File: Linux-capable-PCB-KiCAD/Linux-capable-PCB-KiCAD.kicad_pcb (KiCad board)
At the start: 4 copper layers, 168 parts, among them J1 UART_CONN, J2 GPIO_CONN, J3 USB_A, J4 USB_A, J5 Micro_SD_Card_Det, J6 MIC_DIFF_IN, J7 Barrel_Jack, U1 A33, U10 TPS62130, U11 AP131-25, U12 TPS62130, U13 TPS62130, U2 MMA8425Q_Gsensor, U3 SRV05-4, U4 MIPI_DSI_Raspberry, U5 SRV05-4, U6 SRV05-4, U7 ESP8089, U8 HTQ4G63AFR-PCB, U9 TPS62130, Y1 24MHz, Y2 32.768kHz, Y3 26 MHz

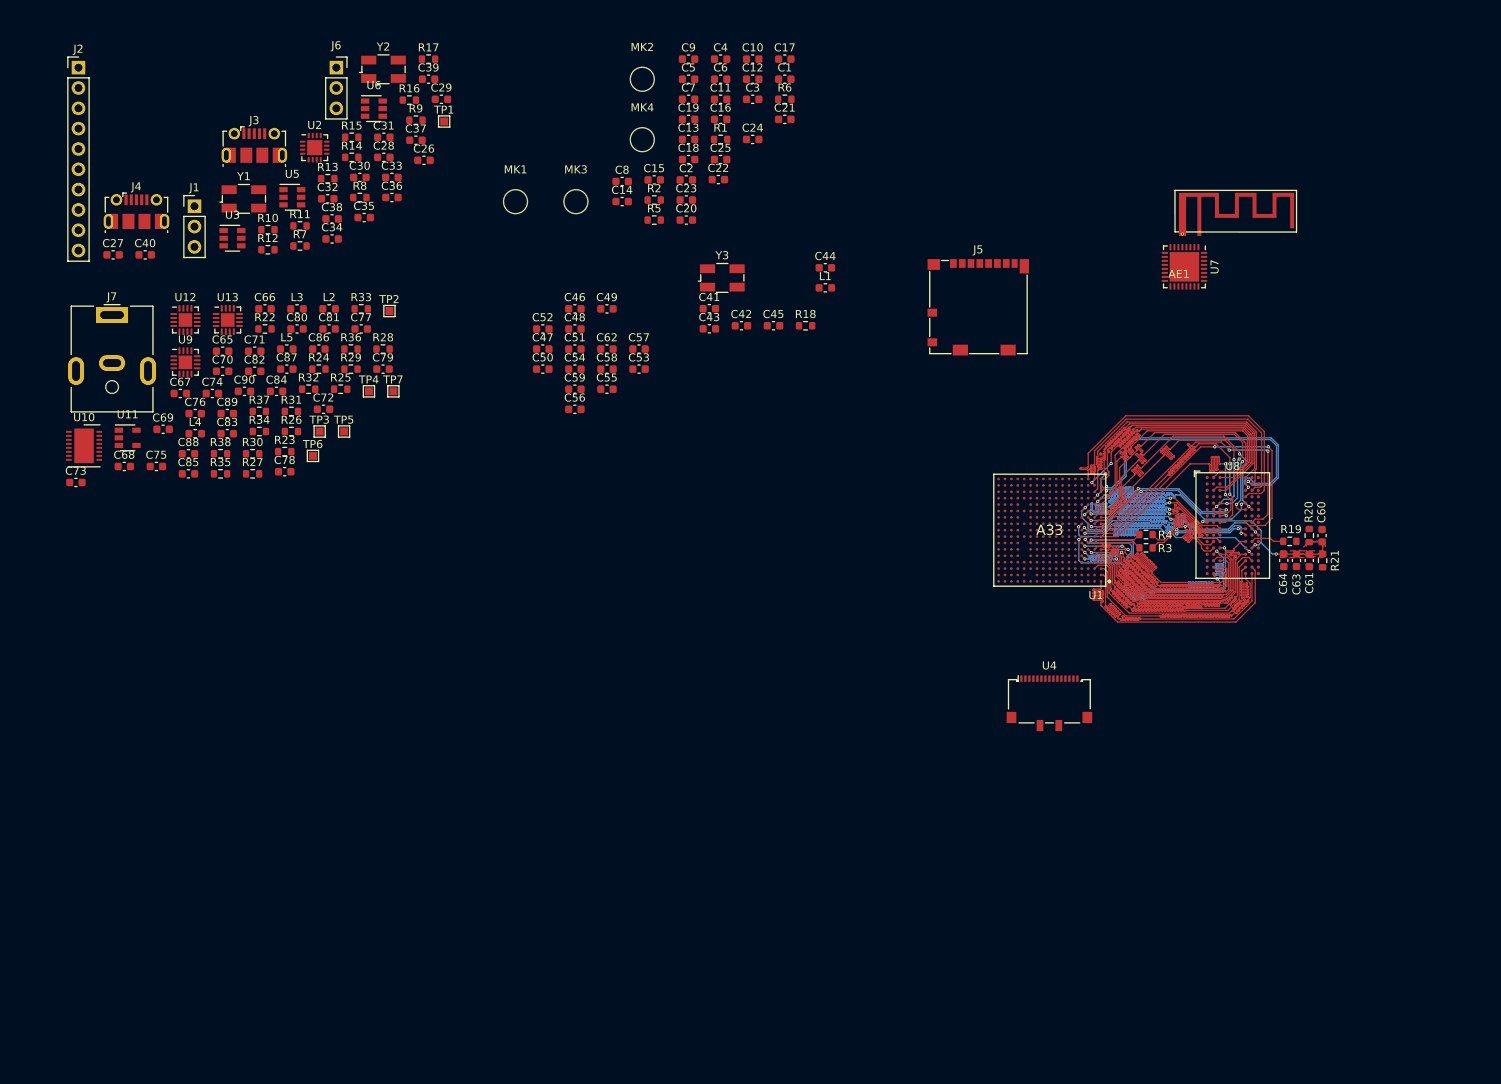
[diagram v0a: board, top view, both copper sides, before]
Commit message: Od kuce
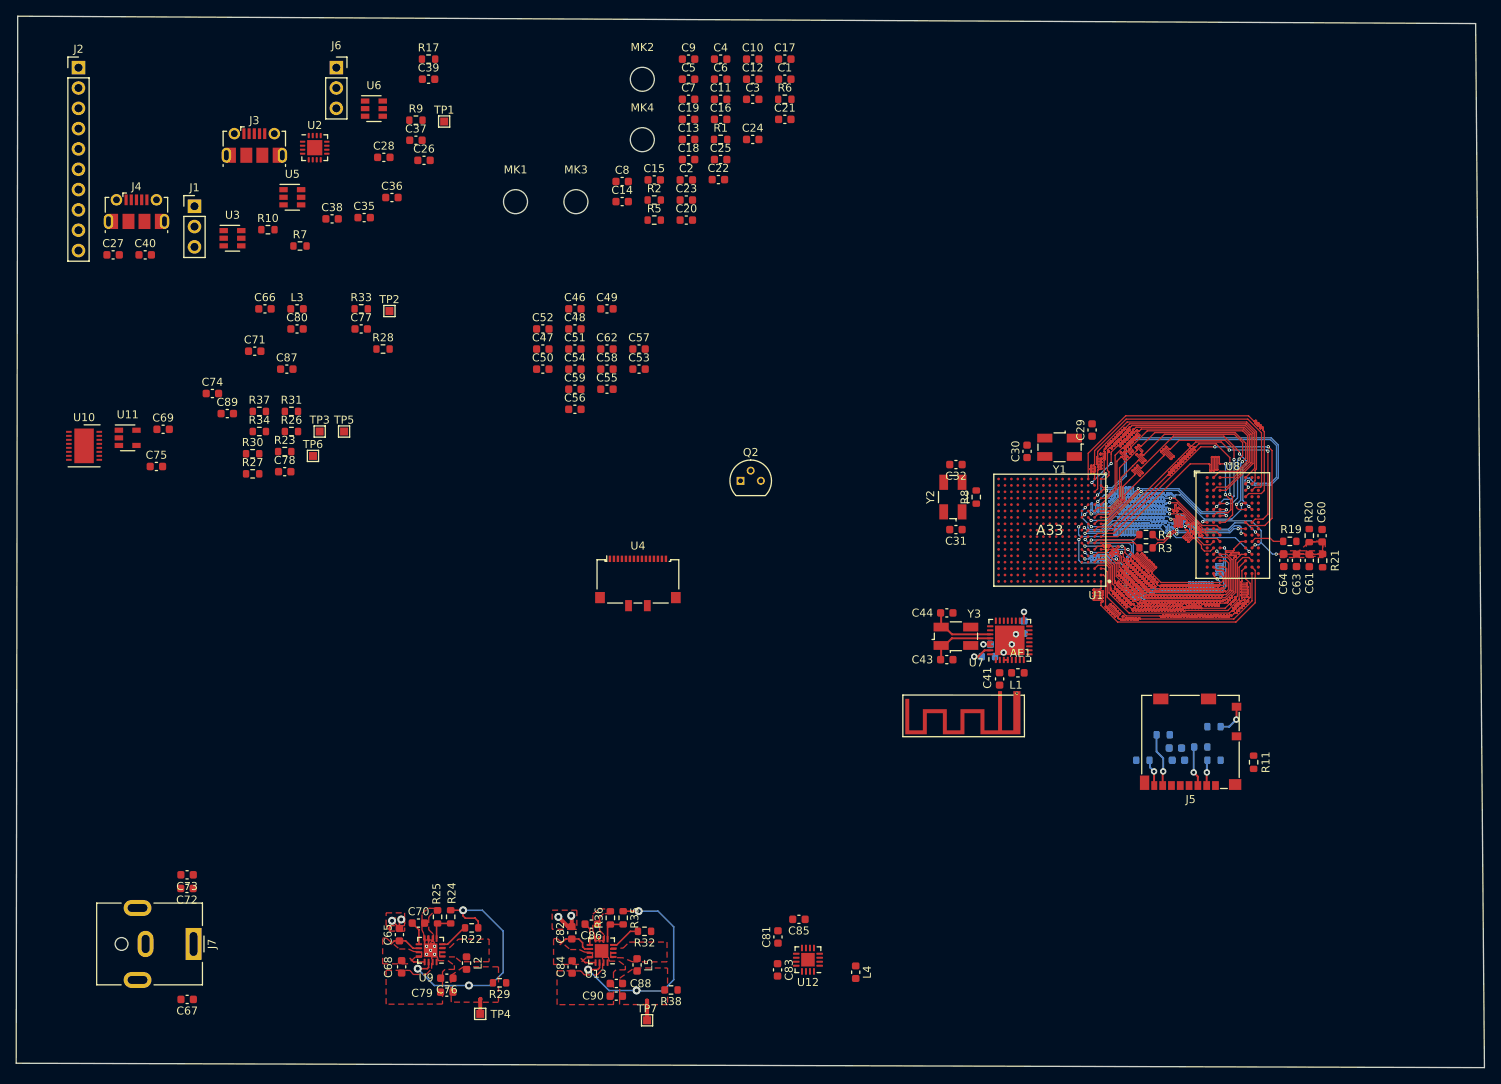
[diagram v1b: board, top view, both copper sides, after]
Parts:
- added Q2: BC547, TO_SOT_Packages_THT:TO-92_Molded_Narrow, F.Cu at (113.8, 72.5)
- C33, C34, C42, C45, R12, R13, R14, R15, R16, R18: moved to B.Cu
- moved R11 136.8 mm to (177.9, 107.7), turned to 90 degrees
- moved R12 134.4 mm to (173.0, 107.4)
- moved R13 130.2 mm to (171.3, 105.8)
- moved R16 127.5 mm to (173.0, 103.3), turned to 180 degrees
- moved R15 125.9 mm to (164.1, 107.4), turned to 180 degrees
- moved R14 124.5 mm to (166.6, 104.3)
- moved C34 124.2 mm to (168.5, 107.4)
- moved C33 121.2 mm to (168.1, 105.9)
- moved U12 111.6 mm to (122.2, 132.4), turned to 180 degrees
- moved Y1 106.6 mm to (153.7, 68.3), turned to 180 degrees
- moved L4 106.5 mm to (128.2, 133.9), turned to -90 degrees
- moved C83 96.0 mm to (118.4, 133.7), turned to -90 degrees
- moved C81 94.5 mm to (118.5, 129.5), turned to 90 degrees
- moved C85 94.5 mm to (121.1, 127.3), turned to 180 degrees
- moved U13 91.7 mm to (96.4, 131.3), turned to 180 degrees
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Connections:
- net /RAM/~CAS renamed /RAM/~{CAS}
- net /RAM/~CKE renamed /RAM/~{CKE}
- net /RAM/~CS renamed /RAM/~{CS}
- net /RAM/~RAS renamed /RAM/~{RAS}
- net /RAM/~RST renamed /RAM/~{RST}
- net /RAM/~WE renamed /RAM/~{WE}
- C29 pad 1: Net-(C29-Pad1) -> unconnected-(C29-Pad1)
- C33 pad 1: Net-(C33-Pad1) -> +3V3
- C34 pad 1: Net-(C33-Pad1) -> +3V3
- J5 pad 4: Net-(C33-Pad1) -> +3V3
- R11 pad 2: Net-(C33-Pad1) -> +3V3
- R12 pad 2: Net-(C33-Pad1) -> +3V3
- R13 pad 2: Net-(C33-Pad1) -> +3V3
- R14 pad 2: Net-(C33-Pad1) -> +3V3
- R15 pad 2: Net-(C33-Pad1) -> +3V3
- R16 pad 2: Net-(C33-Pad1) -> +3V3
- U1 pad A10: Net-(U1-PadA10) -> unconnected-(U1-PadA10)
- U1 pad A11: Net-(U1-PadA11) -> unconnected-(U1-PadA11)
- U1 pad A12: Net-(U1-PadA12) -> unconnected-(U1-PadA12)
- U1 pad A16: Net-(U1-PadA16) -> unconnected-(U1-PadA16)
- U1 pad A2: Net-(U1-PadA2) -> unconnected-(U1-PadA2)
- U1 pad A7: Net-(U1-PadA7) -> unconnected-(U1-PadA7)
- U1 pad A8: Net-(U1-PadA8) -> unconnected-(U1-PadA8)
- U1 pad A9: Net-(U1-PadA9) -> unconnected-(U1-PadA9)
- U1 pad B10: Net-(U1-PadB10) -> unconnected-(U1-PadB10)
- U1 pad B11: Net-(U1-PadB11) -> unconnected-(U1-PadB11)
- U1 pad B16: Net-(U1-PadB16) -> unconnected-(U1-PadB16)
- U1 pad B17: Net-(U1-PadB17) -> unconnected-(U1-PadB17)
- U1 pad B2: Net-(U1-PadB2) -> unconnected-(U1-PadB2)
- U1 pad B7: Net-(U1-PadB7) -> unconnected-(U1-PadB7)
- U1 pad B8: Net-(U1-PadB8) -> unconnected-(U1-PadB8)
- U1 pad B9: Net-(U1-PadB9) -> unconnected-(U1-PadB9)
- U1 pad C10: Net-(U1-PadC10) -> unconnected-(U1-PadC10)
- U1 pad C11: Net-(U1-PadC11) -> unconnected-(U1-PadC11)
- U1 pad C12: Net-(U1-PadC12) -> unconnected-(U1-PadC12)
- U1 pad C13: Net-(U1-PadC13) -> unconnected-(U1-PadC13)
- U1 pad C14: Net-(U1-PadC14) -> unconnected-(U1-PadC14)
- U1 pad C15: Net-(U1-PadC15) -> unconnected-(U1-PadC15)
- U1 pad C16: Net-(U1-PadC16) -> unconnected-(U1-PadC16)
- U1 pad C17: Net-(U1-PadC17) -> unconnected-(U1-PadC17)
- U1 pad C3: Net-(U1-PadC3) -> unconnected-(U1-PadC3)
- U1 pad C4: Net-(U1-PadC4) -> unconnected-(U1-PadC4)
- U1 pad D10: Net-(U1-PadD10) -> unconnected-(U1-PadD10)
- U1 pad D11: Net-(U1-PadD11) -> unconnected-(U1-PadD11)
- U1 pad D12: Net-(U1-PadD12) -> unconnected-(U1-PadD12)
- U1 pad D13: Net-(U1-PadD13) -> unconnected-(U1-PadD13)
- U1 pad D3: Net-(U1-PadD3) -> unconnected-(U1-PadD3)
- U1 pad D4: Net-(U1-PadD4) -> unconnected-(U1-PadD4)
- U1 pad E14: Net-(U1-PadE14) -> unconnected-(U1-PadE14)
- U1 pad E15: Net-(U1-PadE15) -> unconnected-(U1-PadE15)
- U1 pad E16: Net-(U1-PadE16) -> unconnected-(U1-PadE16)
- U1 pad E17: Net-(U1-PadE17) -> unconnected-(U1-PadE17)
- U1 pad F14: Net-(U1-PadF14) -> unconnected-(U1-PadF14)
- U1 pad F15: Net-(U1-PadF15) -> unconnected-(U1-PadF15)
- U1 pad F16: Net-(U1-PadF16) -> unconnected-(U1-PadF16)
- U1 pad F17: Net-(U1-PadF17) -> unconnected-(U1-PadF17)
- U1 pad G15: Net-(U1-PadG15) -> unconnected-(U1-PadG15)
- U1 pad H14: Net-(U1-PadH14) -> unconnected-(U1-PadH14)
- U1 pad H15: Net-(U1-PadH15) -> unconnected-(U1-PadH15)
- U1 pad H16: Net-(U1-PadH16) -> unconnected-(U1-PadH16)
- U1 pad J14: Net-(U1-PadJ14) -> unconnected-(U1-PadJ14)
- U1 pad J15: Net-(U1-PadJ15) -> unconnected-(U1-PadJ15)
- U1 pad J16: Net-(U1-PadJ16) -> unconnected-(U1-PadJ16)
- U1 pad J17: Net-(U1-PadJ17) -> unconnected-(U1-PadJ17)
- U1 pad K14: Net-(U1-PadK14) -> unconnected-(U1-PadK14)
- U1 pad K15: Net-(U1-PadK15) -> unconnected-(U1-PadK15)
- U1 pad L14: Net-(U1-PadL14) -> unconnected-(U1-PadL14)
- U1 pad L15: Net-(U1-PadL15) -> unconnected-(U1-PadL15)
- U1 pad L7: Net-(U1-PadL7) -> unconnected-(U1-PadL7)
- U1 pad M1: d0 -> d[0..15]
- U1 pad M15: Net-(U1-PadM15) -> unconnected-(U1-PadM15)
- U1 pad N15: Net-(U1-PadN15) -> unconnected-(U1-PadN15)
- U1 pad N16: Net-(U1-PadN16) -> unconnected-(U1-PadN16)
- U1 pad N17: Net-(U1-PadN17) -> unconnected-(U1-PadN17)
- U1 pad N5: Net-(U1-PadN5) -> unconnected-(U1-PadN5)
- U1 pad N7: Net-(U1-PadN7) -> unconnected-(U1-PadN7)
- U1 pad P10: Net-(U1-PadP10) -> unconnected-(U1-PadP10)
- U1 pad P11: Net-(U1-PadP11) -> unconnected-(U1-PadP11)
- U1 pad P12: Net-(U1-PadP12) -> unconnected-(U1-PadP12)
- U1 pad P13: Net-(U1-PadP13) -> unconnected-(U1-PadP13)
- U1 pad P14: Net-(U1-PadP14) -> unconnected-(U1-PadP14)
- U1 pad P15: Net-(U1-PadP15) -> unconnected-(U1-PadP15)
- U1 pad P16: Net-(U1-PadP16) -> unconnected-(U1-PadP16)
- U1 pad P6: Net-(U1-PadP6) -> unconnected-(U1-PadP6)
- U1 pad P7: Net-(U1-PadP7) -> unconnected-(U1-PadP7)
- U1 pad P8: Net-(U1-PadP8) -> unconnected-(U1-PadP8)
- U1 pad P9: Net-(U1-PadP9) -> unconnected-(U1-PadP9)
- U1 pad R10: Net-(U1-PadR10) -> unconnected-(U1-PadR10)
- U1 pad R11: Net-(U1-PadR11) -> unconnected-(U1-PadR11)
- U1 pad R12: Net-(U1-PadR12) -> unconnected-(U1-PadR12)
- U1 pad R13: Net-(U1-PadR13) -> unconnected-(U1-PadR13)
- U1 pad R14: Net-(U1-PadR14) -> unconnected-(U1-PadR14)
- U1 pad R15: Net-(U1-PadR15) -> unconnected-(U1-PadR15)
- U1 pad R6: Net-(U1-PadR6) -> unconnected-(U1-PadR6)
- U1 pad R7: Net-(U1-PadR7) -> unconnected-(U1-PadR7)
- U1 pad R8: Net-(U1-PadR8) -> unconnected-(U1-PadR8)
- U1 pad R9: Net-(U1-PadR9) -> unconnected-(U1-PadR9)
- U1 pad T10: Net-(U1-PadT10) -> unconnected-(U1-PadT10)
- U1 pad T11: Net-(U1-PadT11) -> unconnected-(U1-PadT11)
- U1 pad T12: Net-(U1-PadT12) -> unconnected-(U1-PadT12)
- U1 pad T13: Net-(U1-PadT13) -> unconnected-(U1-PadT13)
- U1 pad T14: Net-(U1-PadT14) -> unconnected-(U1-PadT14)
- U1 pad T15: Net-(U1-PadT15) -> unconnected-(U1-PadT15)
- U1 pad T6: Net-(U1-PadT6) -> unconnected-(U1-PadT6)
- U1 pad T7: Net-(U1-PadT7) -> unconnected-(U1-PadT7)
- U1 pad T8: Net-(U1-PadT8) -> unconnected-(U1-PadT8)
- U1 pad T9: Net-(U1-PadT9) -> unconnected-(U1-PadT9)
- U1 pad U10: Net-(U1-PadU10) -> unconnected-(U1-PadU10)
- U1 pad U11: Net-(U1-PadU11) -> unconnected-(U1-PadU11)
- U1 pad U12: Net-(U1-PadU12) -> unconnected-(U1-PadU12)
- U1 pad U13: /A33_GPIO/VBUS_~EN -> /A33_GPIO/VBUS_~{EN}
- U1 pad U14: Net-(U1-PadU14) -> unconnected-(U1-PadU14)
- U1 pad U15: Net-(U1-PadU15) -> unconnected-(U1-PadU15)
- U1 pad U6: Net-(U1-PadU6) -> unconnected-(U1-PadU6)
- U1 pad U7: Net-(U1-PadU7) -> unconnected-(U1-PadU7)
- U1 pad U8: Net-(U1-PadU8) -> unconnected-(U1-PadU8)
- U1 pad U9: Net-(U1-PadU9) -> unconnected-(U1-PadU9)
- U2 pad 13: Net-(U2-Pad13) -> unconnected-(U2-Pad13)
- U2 pad 15: Net-(U2-Pad15) -> unconnected-(U2-Pad15)
- U2 pad 16: Net-(U2-Pad16) -> unconnected-(U2-Pad16)
- U2 pad 3: Net-(U2-Pad3) -> unconnected-(U2-Pad3)
- U2 pad 8: Net-(U2-Pad8) -> unconnected-(U2-Pad8)
- U7 pad 10: Net-(U7-Pad10) -> unconnected-(U7-Pad10)
- U7 pad 12: Net-(U7-Pad12) -> unconnected-(U7-Pad12)
- U7 pad 13: Net-(U7-Pad13) -> unconnected-(U7-Pad13)
- U7 pad 14: Net-(U7-Pad14) -> unconnected-(U7-Pad14)
- U7 pad 15: Net-(U7-Pad15) -> unconnected-(U7-Pad15)
- U7 pad 16: Net-(U7-Pad16) -> unconnected-(U7-Pad16)
- U7 pad 24: Net-(U7-Pad24) -> unconnected-(U7-Pad24)
- U7 pad 25: Net-(U7-Pad25) -> unconnected-(U7-Pad25)
- U7 pad 26: Net-(U7-Pad26) -> unconnected-(U7-Pad26)
- U7 pad 32: Net-(U7-Pad32) -> unconnected-(U7-Pad32)
- U7 pad 5: Net-(U7-Pad5) -> unconnected-(U7-Pad5)
- U7 pad 6: Net-(U7-Pad6) -> unconnected-(U7-Pad6)
- U7 pad 8: Net-(U7-Pad8) -> unconnected-(U7-Pad8)
- U7 pad 9: Net-(U7-Pad9) -> unconnected-(U7-Pad9)
- U8 pad J1: Net-(U8-PadJ1) -> unconnected-(U8-PadJ1)
- U8 pad J9: Net-(U8-PadJ9) -> unconnected-(U8-PadJ9)
- U8 pad L1: Net-(U8-PadL1) -> unconnected-(U8-PadL1)
- U8 pad L9: Net-(U8-PadL9) -> unconnected-(U8-PadL9)
- U8 pad M7: Net-(U8-PadM7) -> unconnected-(U8-PadM7)
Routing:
- net d[0..15]: track 0.00 -> 38.0 mm, vias 0 -> 2
- net d0: track 38.0 -> 0.00 mm, vias 2 -> 0
- net Net-(C76-Pad1): track 0.00 -> 32.8 mm, vias 0 -> 3
- net Net-(C88-Pad1): track 0.00 -> 30.8 mm, vias 0 -> 3
- net GND: track 0.00 -> 19.0 mm, vias 0 -> 12
- net +5V: track 0.00 -> 12.9 mm
- net Net-(C44-Pad2): track 0.00 -> 8.31 mm
- net Net-(C43-Pad2): track 0.00 -> 8.30 mm
- net /A33_GPIO/SD_DAT0: track 0.00 -> 6.71 mm, vias 0 -> 1
- net /A33_GPIO/SD_CMD: track 0.00 -> 5.06 mm, vias 0 -> 1
- net +3V3: track 0.00 -> 4.99 mm, vias 0 -> 2
- net /A33_GPIO/SD_DET: track 0.00 -> 3.95 mm, vias 0 -> 1
- net Net-(R32-Pad2): track 0.00 -> 3.79 mm
- net Net-(R22-Pad2): track 0.00 -> 3.69 mm
- net Net-(R35-Pad2): track 0.00 -> 3.62 mm
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- added copper zone on F.Cu, net +5V
- added copper zone on F.Cu, net GND
- added copper zone on F.Cu, net Net-(C76-Pad1)
- added copper zone on F.Cu, net Net-(C88-Pad1)
- added copper zone on F.Cu, net Net-(L2-Pad1)
- added copper zone on F.Cu, net Net-(L5-Pad1)
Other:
- board outline added: 183.5 x 131.4 mm
- net class Default removed
- net class Outer_small removed
- net class Power removed

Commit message: Revert "Od kuce"
This reverts commit 2bece482254f98a379437a0618b8cb6327aa6629.
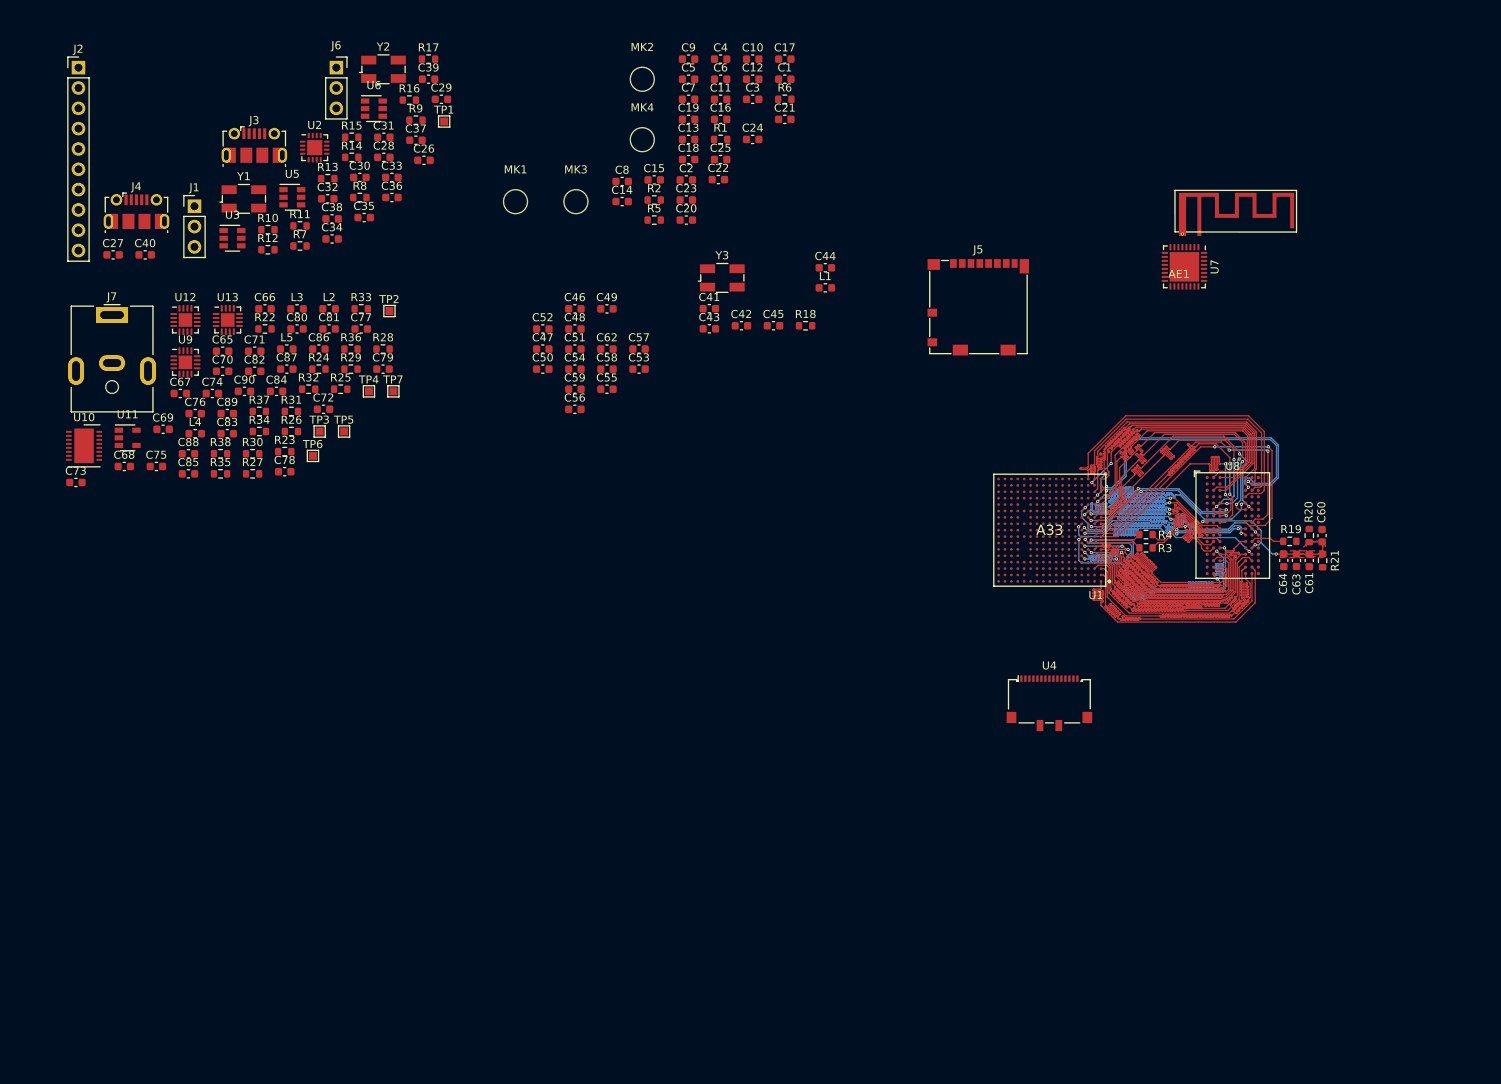
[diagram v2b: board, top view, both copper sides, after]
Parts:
- removed Q2: BC547, TO_SOT_Packages_THT:TO-92_Molded_Narrow
- C33, C34, C42, C45, R12, R13, R14, R15, R16, R18: moved to F.Cu
- moved R11 136.8 mm to (58.7, 40.7), turned to 0 degrees
- moved R12 134.4 mm to (54.7, 43.6)
- moved R13 130.2 mm to (62.2, 34.8)
- moved R16 127.5 mm to (72.4, 24.9), turned to 0 degrees
- moved R15 125.9 mm to (65.2, 29.6), turned to 0 degrees
- moved R14 124.5 mm to (65.2, 32.1)
- moved C34 124.2 mm to (62.7, 42.3)
- moved C33 121.2 mm to (70.2, 34.6)
- moved U12 111.6 mm to (44.4, 52.4), turned to 0 degrees
- moved Y1 106.6 mm to (51.7, 37.3), turned to 0 degrees
- moved L4 106.5 mm to (45.6, 66.6), turned to 0 degrees
- moved C83 96.0 mm to (49.6, 66.6), turned to 0 degrees
- moved C81 94.5 mm to (62.4, 53.5), turned to 0 degrees
- moved C85 94.5 mm to (44.8, 71.6), turned to 0 degrees
- moved U13 91.7 mm to (49.7, 52.4), turned to 0 degrees
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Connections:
- net /RAM/~{CAS} renamed /RAM/~CAS
- net /RAM/~{CKE} renamed /RAM/~CKE
- net /RAM/~{CS} renamed /RAM/~CS
- net /RAM/~{RAS} renamed /RAM/~RAS
- net /RAM/~{RST} renamed /RAM/~RST
- net /RAM/~{WE} renamed /RAM/~WE
- C29 pad 1: unconnected-(C29-Pad1) -> Net-(C29-Pad1)
- C33 pad 1: +3V3 -> Net-(C33-Pad1)
- C34 pad 1: +3V3 -> Net-(C33-Pad1)
- J5 pad 4: +3V3 -> Net-(C33-Pad1)
- R11 pad 2: +3V3 -> Net-(C33-Pad1)
- R12 pad 2: +3V3 -> Net-(C33-Pad1)
- R13 pad 2: +3V3 -> Net-(C33-Pad1)
- R14 pad 2: +3V3 -> Net-(C33-Pad1)
- R15 pad 2: +3V3 -> Net-(C33-Pad1)
- R16 pad 2: +3V3 -> Net-(C33-Pad1)
- U1 pad A10: unconnected-(U1-PadA10) -> Net-(U1-PadA10)
- U1 pad A11: unconnected-(U1-PadA11) -> Net-(U1-PadA11)
- U1 pad A12: unconnected-(U1-PadA12) -> Net-(U1-PadA12)
- U1 pad A16: unconnected-(U1-PadA16) -> Net-(U1-PadA16)
- U1 pad A2: unconnected-(U1-PadA2) -> Net-(U1-PadA2)
- U1 pad A7: unconnected-(U1-PadA7) -> Net-(U1-PadA7)
- U1 pad A8: unconnected-(U1-PadA8) -> Net-(U1-PadA8)
- U1 pad A9: unconnected-(U1-PadA9) -> Net-(U1-PadA9)
- U1 pad B10: unconnected-(U1-PadB10) -> Net-(U1-PadB10)
- U1 pad B11: unconnected-(U1-PadB11) -> Net-(U1-PadB11)
- U1 pad B16: unconnected-(U1-PadB16) -> Net-(U1-PadB16)
- U1 pad B17: unconnected-(U1-PadB17) -> Net-(U1-PadB17)
- U1 pad B2: unconnected-(U1-PadB2) -> Net-(U1-PadB2)
- U1 pad B7: unconnected-(U1-PadB7) -> Net-(U1-PadB7)
- U1 pad B8: unconnected-(U1-PadB8) -> Net-(U1-PadB8)
- U1 pad B9: unconnected-(U1-PadB9) -> Net-(U1-PadB9)
- U1 pad C10: unconnected-(U1-PadC10) -> Net-(U1-PadC10)
- U1 pad C11: unconnected-(U1-PadC11) -> Net-(U1-PadC11)
- U1 pad C12: unconnected-(U1-PadC12) -> Net-(U1-PadC12)
- U1 pad C13: unconnected-(U1-PadC13) -> Net-(U1-PadC13)
- U1 pad C14: unconnected-(U1-PadC14) -> Net-(U1-PadC14)
- U1 pad C15: unconnected-(U1-PadC15) -> Net-(U1-PadC15)
- U1 pad C16: unconnected-(U1-PadC16) -> Net-(U1-PadC16)
- U1 pad C17: unconnected-(U1-PadC17) -> Net-(U1-PadC17)
- U1 pad C3: unconnected-(U1-PadC3) -> Net-(U1-PadC3)
- U1 pad C4: unconnected-(U1-PadC4) -> Net-(U1-PadC4)
- U1 pad D10: unconnected-(U1-PadD10) -> Net-(U1-PadD10)
- U1 pad D11: unconnected-(U1-PadD11) -> Net-(U1-PadD11)
- U1 pad D12: unconnected-(U1-PadD12) -> Net-(U1-PadD12)
- U1 pad D13: unconnected-(U1-PadD13) -> Net-(U1-PadD13)
- U1 pad D3: unconnected-(U1-PadD3) -> Net-(U1-PadD3)
- U1 pad D4: unconnected-(U1-PadD4) -> Net-(U1-PadD4)
- U1 pad E14: unconnected-(U1-PadE14) -> Net-(U1-PadE14)
- U1 pad E15: unconnected-(U1-PadE15) -> Net-(U1-PadE15)
- U1 pad E16: unconnected-(U1-PadE16) -> Net-(U1-PadE16)
- U1 pad E17: unconnected-(U1-PadE17) -> Net-(U1-PadE17)
- U1 pad F14: unconnected-(U1-PadF14) -> Net-(U1-PadF14)
- U1 pad F15: unconnected-(U1-PadF15) -> Net-(U1-PadF15)
- U1 pad F16: unconnected-(U1-PadF16) -> Net-(U1-PadF16)
- U1 pad F17: unconnected-(U1-PadF17) -> Net-(U1-PadF17)
- U1 pad G15: unconnected-(U1-PadG15) -> Net-(U1-PadG15)
- U1 pad H14: unconnected-(U1-PadH14) -> Net-(U1-PadH14)
- U1 pad H15: unconnected-(U1-PadH15) -> Net-(U1-PadH15)
- U1 pad H16: unconnected-(U1-PadH16) -> Net-(U1-PadH16)
- U1 pad J14: unconnected-(U1-PadJ14) -> Net-(U1-PadJ14)
- U1 pad J15: unconnected-(U1-PadJ15) -> Net-(U1-PadJ15)
- U1 pad J16: unconnected-(U1-PadJ16) -> Net-(U1-PadJ16)
- U1 pad J17: unconnected-(U1-PadJ17) -> Net-(U1-PadJ17)
- U1 pad K14: unconnected-(U1-PadK14) -> Net-(U1-PadK14)
- U1 pad K15: unconnected-(U1-PadK15) -> Net-(U1-PadK15)
- U1 pad L14: unconnected-(U1-PadL14) -> Net-(U1-PadL14)
- U1 pad L15: unconnected-(U1-PadL15) -> Net-(U1-PadL15)
- U1 pad L7: unconnected-(U1-PadL7) -> Net-(U1-PadL7)
- U1 pad M1: d[0..15] -> d0
- U1 pad M15: unconnected-(U1-PadM15) -> Net-(U1-PadM15)
- U1 pad N15: unconnected-(U1-PadN15) -> Net-(U1-PadN15)
- U1 pad N16: unconnected-(U1-PadN16) -> Net-(U1-PadN16)
- U1 pad N17: unconnected-(U1-PadN17) -> Net-(U1-PadN17)
- U1 pad N5: unconnected-(U1-PadN5) -> Net-(U1-PadN5)
- U1 pad N7: unconnected-(U1-PadN7) -> Net-(U1-PadN7)
- U1 pad P10: unconnected-(U1-PadP10) -> Net-(U1-PadP10)
- U1 pad P11: unconnected-(U1-PadP11) -> Net-(U1-PadP11)
- U1 pad P12: unconnected-(U1-PadP12) -> Net-(U1-PadP12)
- U1 pad P13: unconnected-(U1-PadP13) -> Net-(U1-PadP13)
- U1 pad P14: unconnected-(U1-PadP14) -> Net-(U1-PadP14)
- U1 pad P15: unconnected-(U1-PadP15) -> Net-(U1-PadP15)
- U1 pad P16: unconnected-(U1-PadP16) -> Net-(U1-PadP16)
- U1 pad P6: unconnected-(U1-PadP6) -> Net-(U1-PadP6)
- U1 pad P7: unconnected-(U1-PadP7) -> Net-(U1-PadP7)
- U1 pad P8: unconnected-(U1-PadP8) -> Net-(U1-PadP8)
- U1 pad P9: unconnected-(U1-PadP9) -> Net-(U1-PadP9)
- U1 pad R10: unconnected-(U1-PadR10) -> Net-(U1-PadR10)
- U1 pad R11: unconnected-(U1-PadR11) -> Net-(U1-PadR11)
- U1 pad R12: unconnected-(U1-PadR12) -> Net-(U1-PadR12)
- U1 pad R13: unconnected-(U1-PadR13) -> Net-(U1-PadR13)
- U1 pad R14: unconnected-(U1-PadR14) -> Net-(U1-PadR14)
- U1 pad R15: unconnected-(U1-PadR15) -> Net-(U1-PadR15)
- U1 pad R6: unconnected-(U1-PadR6) -> Net-(U1-PadR6)
- U1 pad R7: unconnected-(U1-PadR7) -> Net-(U1-PadR7)
- U1 pad R8: unconnected-(U1-PadR8) -> Net-(U1-PadR8)
- U1 pad R9: unconnected-(U1-PadR9) -> Net-(U1-PadR9)
- U1 pad T10: unconnected-(U1-PadT10) -> Net-(U1-PadT10)
- U1 pad T11: unconnected-(U1-PadT11) -> Net-(U1-PadT11)
- U1 pad T12: unconnected-(U1-PadT12) -> Net-(U1-PadT12)
- U1 pad T13: unconnected-(U1-PadT13) -> Net-(U1-PadT13)
- U1 pad T14: unconnected-(U1-PadT14) -> Net-(U1-PadT14)
- U1 pad T15: unconnected-(U1-PadT15) -> Net-(U1-PadT15)
- U1 pad T6: unconnected-(U1-PadT6) -> Net-(U1-PadT6)
- U1 pad T7: unconnected-(U1-PadT7) -> Net-(U1-PadT7)
- U1 pad T8: unconnected-(U1-PadT8) -> Net-(U1-PadT8)
- U1 pad T9: unconnected-(U1-PadT9) -> Net-(U1-PadT9)
- U1 pad U10: unconnected-(U1-PadU10) -> Net-(U1-PadU10)
- U1 pad U11: unconnected-(U1-PadU11) -> Net-(U1-PadU11)
- U1 pad U12: unconnected-(U1-PadU12) -> Net-(U1-PadU12)
- U1 pad U13: /A33_GPIO/VBUS_~{EN} -> /A33_GPIO/VBUS_~EN
- U1 pad U14: unconnected-(U1-PadU14) -> Net-(U1-PadU14)
- U1 pad U15: unconnected-(U1-PadU15) -> Net-(U1-PadU15)
- U1 pad U6: unconnected-(U1-PadU6) -> Net-(U1-PadU6)
- U1 pad U7: unconnected-(U1-PadU7) -> Net-(U1-PadU7)
- U1 pad U8: unconnected-(U1-PadU8) -> Net-(U1-PadU8)
- U1 pad U9: unconnected-(U1-PadU9) -> Net-(U1-PadU9)
- U2 pad 13: unconnected-(U2-Pad13) -> Net-(U2-Pad13)
- U2 pad 15: unconnected-(U2-Pad15) -> Net-(U2-Pad15)
- U2 pad 16: unconnected-(U2-Pad16) -> Net-(U2-Pad16)
- U2 pad 3: unconnected-(U2-Pad3) -> Net-(U2-Pad3)
- U2 pad 8: unconnected-(U2-Pad8) -> Net-(U2-Pad8)
- U7 pad 10: unconnected-(U7-Pad10) -> Net-(U7-Pad10)
- U7 pad 12: unconnected-(U7-Pad12) -> Net-(U7-Pad12)
- U7 pad 13: unconnected-(U7-Pad13) -> Net-(U7-Pad13)
- U7 pad 14: unconnected-(U7-Pad14) -> Net-(U7-Pad14)
- U7 pad 15: unconnected-(U7-Pad15) -> Net-(U7-Pad15)
- U7 pad 16: unconnected-(U7-Pad16) -> Net-(U7-Pad16)
- U7 pad 24: unconnected-(U7-Pad24) -> Net-(U7-Pad24)
- U7 pad 25: unconnected-(U7-Pad25) -> Net-(U7-Pad25)
- U7 pad 26: unconnected-(U7-Pad26) -> Net-(U7-Pad26)
- U7 pad 32: unconnected-(U7-Pad32) -> Net-(U7-Pad32)
- U7 pad 5: unconnected-(U7-Pad5) -> Net-(U7-Pad5)
- U7 pad 6: unconnected-(U7-Pad6) -> Net-(U7-Pad6)
- U7 pad 8: unconnected-(U7-Pad8) -> Net-(U7-Pad8)
- U7 pad 9: unconnected-(U7-Pad9) -> Net-(U7-Pad9)
- U8 pad J1: unconnected-(U8-PadJ1) -> Net-(U8-PadJ1)
- U8 pad J9: unconnected-(U8-PadJ9) -> Net-(U8-PadJ9)
- U8 pad L1: unconnected-(U8-PadL1) -> Net-(U8-PadL1)
- U8 pad L9: unconnected-(U8-PadL9) -> Net-(U8-PadL9)
- U8 pad M7: unconnected-(U8-PadM7) -> Net-(U8-PadM7)
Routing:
- net d[0..15]: track 38.0 -> 0.00 mm, vias 2 -> 0
- net d0: track 0.00 -> 38.0 mm, vias 0 -> 2
- net Net-(C76-Pad1): track 32.8 -> 0.00 mm, vias 3 -> 0
- net Net-(C88-Pad1): track 30.8 -> 0.00 mm, vias 3 -> 0
- net GND: track 19.0 -> 0.00 mm, vias 12 -> 0
- net +5V: track 12.9 -> 0.00 mm
- net Net-(C44-Pad2): track 8.31 -> 0.00 mm
- net Net-(C43-Pad2): track 8.30 -> 0.00 mm
- net /A33_GPIO/SD_DAT0: track 6.71 -> 0.00 mm, vias 1 -> 0
- net /A33_GPIO/SD_CMD: track 5.06 -> 0.00 mm, vias 1 -> 0
- net +3V3: track 4.99 -> 0.00 mm, vias 2 -> 0
- net /A33_GPIO/SD_DET: track 3.95 -> 0.00 mm, vias 1 -> 0
- net Net-(R32-Pad2): track 3.79 -> 0.00 mm
- net Net-(R22-Pad2): track 3.69 -> 0.00 mm
- net Net-(R35-Pad2): track 3.62 -> 0.00 mm
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- removed copper zone on F.Cu, net +5V
- removed copper zone on F.Cu, net GND
- removed copper zone on F.Cu, net Net-(C76-Pad1)
- removed copper zone on F.Cu, net Net-(C88-Pad1)
- removed copper zone on F.Cu, net Net-(L2-Pad1)
- removed copper zone on F.Cu, net Net-(L5-Pad1)
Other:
- board outline removed
- net class Default added: clearance 0.12, trace_width 0.25, via_dia 0.8, via_drill 0.4
- net class Outer_small added: clearance 0.1, trace_width 0.1, via_dia 0.4, via_drill 0.2
- net class Power added: clearance 0.2, trace_width 1, via_dia 0.8, via_drill 0.6
